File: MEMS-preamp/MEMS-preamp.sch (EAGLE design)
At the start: 23 parts, among them IC1 OPA2134PA, Q4 2N5484

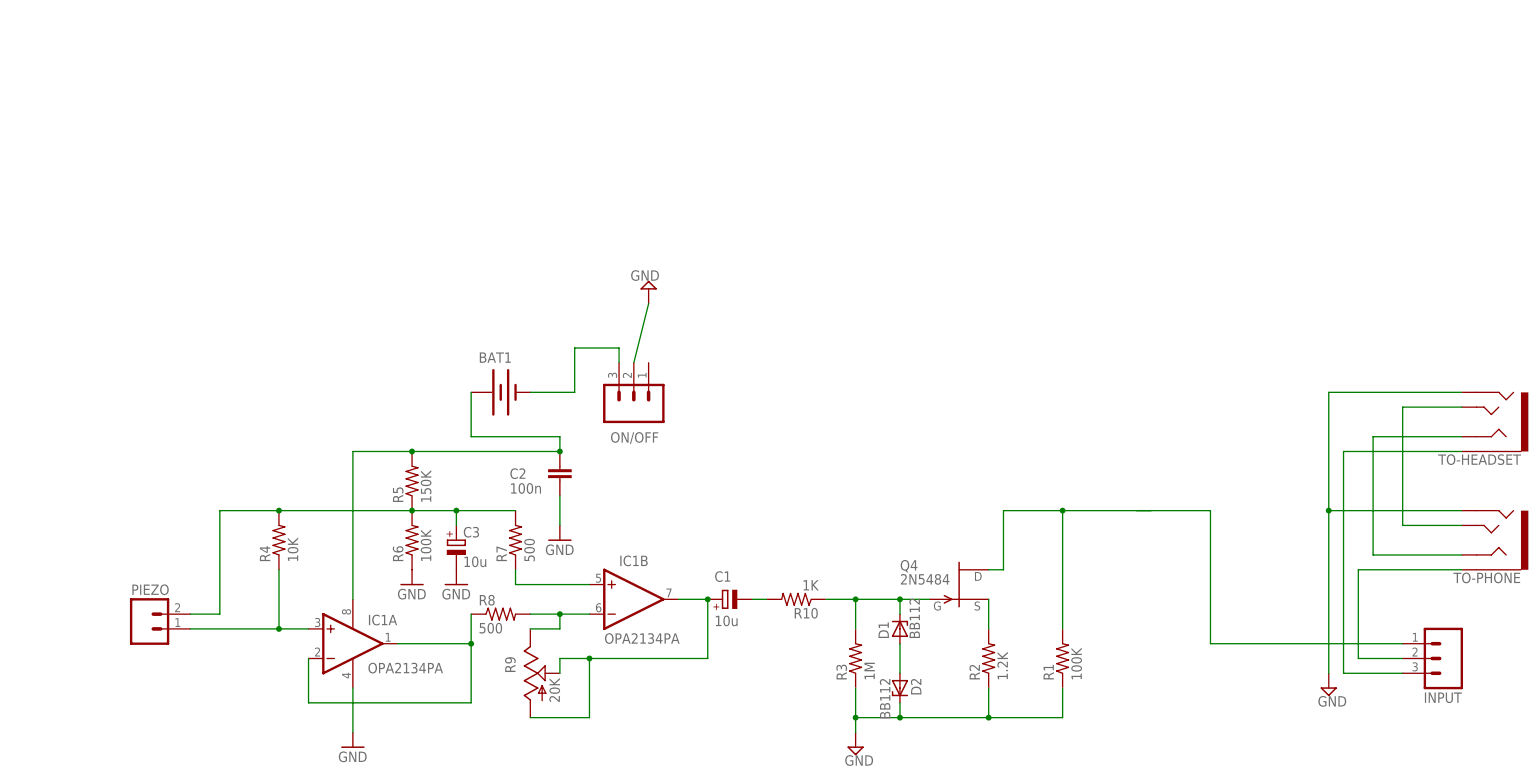
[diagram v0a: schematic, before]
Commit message: changes to TeensyLC midi
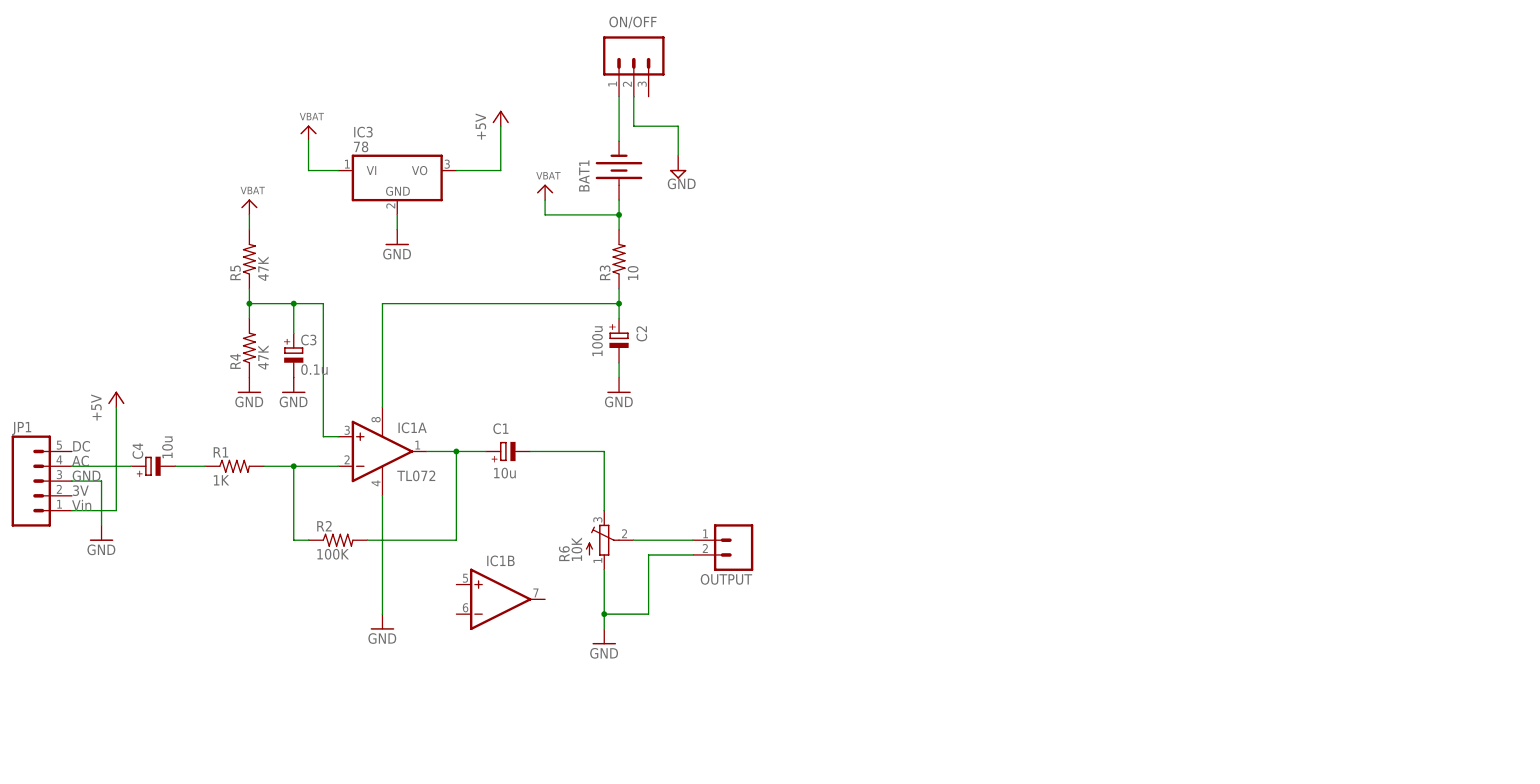
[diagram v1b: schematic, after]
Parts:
- removed D1, D2: BB112, diode:ZENER-DIODEZD-2.5
- removed INPUT: (no value), Daniel:M03SINGLE-POLE-DOUBLE-THROW
- removed PIEZO: (no value), SparkFun-Connectors:M02LOCK
- removed Q4: 2N5484, transistor-fet:2N5484
- removed R10: 1K, CMU-ArtFab:R-US_0204/2V
- removed R7, R8: 500, CMU-ArtFab:R-US_0204/2V
- removed R9: 20K, CMU-ArtFab:TRIMPOT-BOURNS
- removed TO-HEADSET, TO-PHONE: AUDIO-JACK3LGPADS, Daniel:AUDIO-JACK3LGPADS
- added C4: 10u, rcl:CPOL-EUE2.5-5
- added IC3: 78, CMU-ArtFab:78
- added JP1: (no value), SparkFun-Connectors:M05LOCK
- added OUTPUT: (no value), SparkFun-Connectors:M02LOCK
- C2: value 100n -> 100u; device rcl:C-EU025-025X050 -> rcl:CPOL-EUE2.5-5
- C3: value 10u -> 0.1u
- IC1: IC_NAME (none) -> TL072
- R1: value 100K -> 1K; device CMU-ArtFab:R-US_0204/2V -> CMU-ArtFab:R-US_0204/5
- R2: value 1.2K -> 100K; device CMU-ArtFab:R-US_0204/2V -> CMU-ArtFab:R-US_0204/5
- R3: value 1M -> 10; device CMU-ArtFab:R-US_0204/2V -> CMU-ArtFab:R-US_0204/5
- R4: value 10K -> 47K; device CMU-ArtFab:R-US_0204/2V -> CMU-ArtFab:R-US_0204/5
- R5: value 150K -> 47K; device CMU-ArtFab:R-US_0204/2V -> CMU-ArtFab:R-US_0204/5
- R6: value 100K -> 10K; device CMU-ArtFab:R-US_0204/2V -> adafruit:TRIMPOT3386
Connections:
- removed net N$10: D1.C, Q4.G, R10.1, R3.2
- removed net N$11: C1.-, R10.2
- removed net N$12: INPUT.3, TO-HEADSET.EARTH
- removed net N$13: TO-HEADSET.TIP, TO-PHONE.TIP
- removed net N$14: IC1A.-IN, IC1A.OUT, R8.1
- removed net N$15: TO-HEADSET.RING1, TO-PHONE.RING1
- removed net TO-PHONE: INPUT.2, TO-PHONE.EARTH
- removed net V9V: BAT1.+, C2.2, IC1A.V+, R5.2
- removed net `DEL: INPUT.1, Q4.D, R1.2
- new net +5V: IC3.VO, JP1.1
- new net N$4: C4.-, R1.1
- new net VBAT: BAT1.+, IC3.VI, R3.2, R5.2
- net GND: now also C2.-, IC3.GND, JP1.3, OUTPUT.2, R4.1, R6.A; no longer C2.1, D2.C, R1.1, R2.1, R3.1, R6.1, TO-HEADSET.RING2, TO-PHONE.RING2
- net N$1: now also C2.+, IC1A.V+, R3.1; no longer D1.A, D2.A
- net N$2: now also ON/OFF.1; no longer ON/OFF.3
- net N$3: now also C4.+, JP1.4; no longer Q4.S, R2.2
- net N$5: now also IC1A.-IN, R1.2, R2.1; no longer IC1B.+IN, R7.1
- net N$6: now also C1.-, R6.E; no longer C1.+, IC1B.OUT, R9.IN, R9.WIPER
- net N$7: now also OUTPUT.1, R6.S; no longer IC1B.-IN, R8.2, R9.OUT
- net N$8: now also IC1A.+IN; no longer PIEZO.2, R6.2, R7.2
- net N$9: now also C1.+, IC1A.OUT, R2.2; no longer IC1A.+IN, PIEZO.1, R4.1
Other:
- moved on the sheet: BAT1, C1, C3, IC1A, IC1B, ON/OFF, R1, R2, R3, R4, R5
